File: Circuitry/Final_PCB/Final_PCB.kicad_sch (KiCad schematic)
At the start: 110 parts, among them Q1 Q_Dual_NMOS_S1G1D2S2G2D1, Q2 Q_Dual_NMOS_S1G1D2S2G2D1, Q3 Q_Dual_NMOS_S1G1D2S2G2D1, Q4 Q_Dual_NMOS_S1G1D2S2G2D1, Q5 Q_Dual_NMOS_S1G1D2S2G2D1, Q6 Q_Dual_NMOS_S1G1D2S2G2D1, Q7 Q_Dual_NMOS_S1G1D2S2G2D1, Q8 Q_Dual_NMOS_S1G1D2S2G2D1, SW1 SW_SPST, SW2 SW_SPST

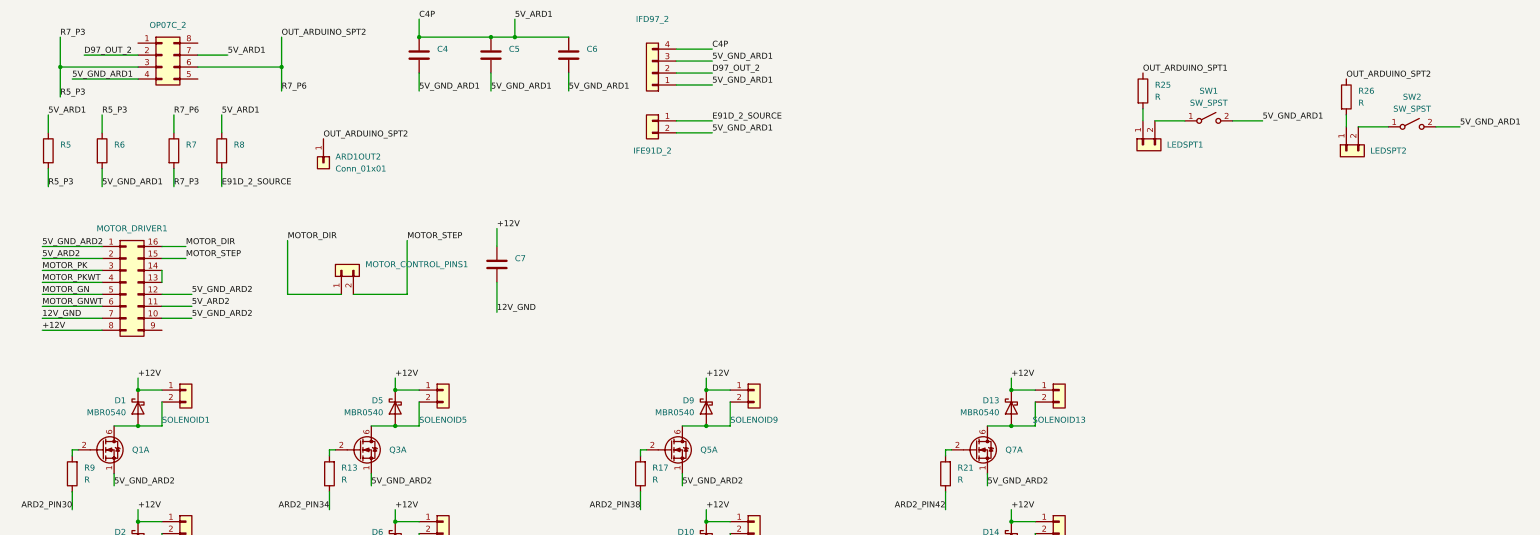
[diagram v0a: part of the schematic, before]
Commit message: final pcb and code updates
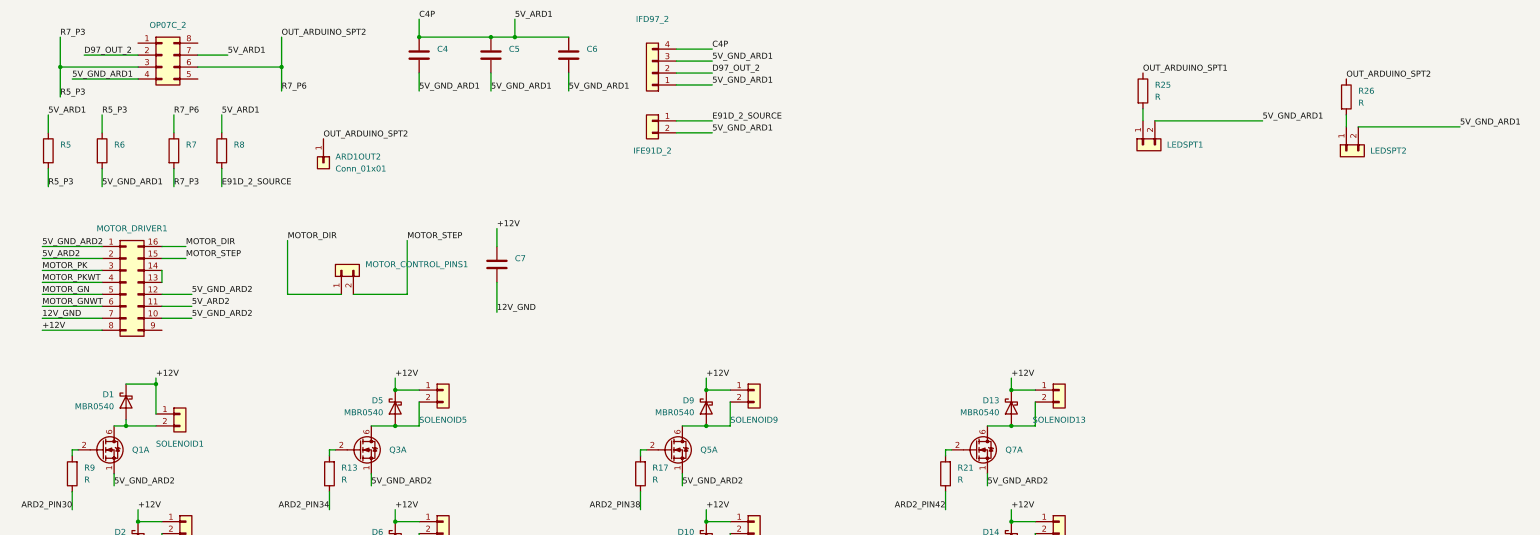
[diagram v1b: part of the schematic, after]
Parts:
- removed SW1, SW2: SW_SPST, Resistor_THT:R_Axial_DIN0207_L6.3mm_D2.5mm_P5.08mm_Vertical, symbol Switch:SW_SPST
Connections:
- net 12V_GND: now also LEDSPT1.2 (Pin_2), LEDSPT2.2 (Pin_2)
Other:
- moved on the sheet: SOLENOID1
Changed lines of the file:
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@@
   (junction (at 372.11 332.74) (diameter 0) (color 0 0 0 0)
   )
+  (junction (at 313.69 247.65) (diameter 0) (color 0 0 0 0)
+  )
   (junction (at 372.11 304.8) (diameter 0) (color 0 0 0 0)
   )
@@
   (junction (at 370.84 247.65) (diameter 0) (color 0 0 0 0)
   )
-  (junction (at 316.23 247.65) (diameter 0) (color 0 0 0 0)
-  )
-  (junction (at 316.23 240.03) (diameter 0) (color 0 0 0 0)
-  )
   (junction (at 502.92 304.8) (diameter 0) (color 0 0 0 0)
   )
@@
   (junction (at 436.88 247.65) (diameter 0) (color 0 0 0 0)
   )
+  (junction (at 320.04 238.76) (diameter 0) (color 0 0 0 0)
+  )
   (junction (at 519.43 143.51) (diameter 0) (color 0 0 0 0)
   )
@@
     (stroke (width 0) (type default))
   )
+  (wire (pts (xy 313.69 238.76) (xy 320.04 238.76))
+    (stroke (width 0) (type default))
+  )
   (wire (pts (xy 295.91 222.25) (xy 308.61 222.25))
     (stroke (width 0) (type default))
@@
     (stroke (width 0) (type default))
   )
-  (wire (pts (xy 316.23 240.03) (xy 321.31 240.03))
+  (wire (pts (xy 320.04 238.76) (xy 320.04 245.11))
     (stroke (width 0) (type default))
   )
@@
     (stroke (width 0) (type default))
   )
-  (wire (pts (xy 548.64 182.88) (xy 554.99 182.88))
-    (stroke (width 0) (type default))
-  )
   (wire (pts (xy 317.5 304.8) (xy 322.58 304.8))
     (stroke (width 0) (type default))
@@
     (stroke (width 0) (type default))
   )
-  (wire (pts (xy 581.66 184.15) (xy 575.31 184.15))
-    (stroke (width 0) (type default))
-  )
   (wire (pts (xy 347.98 123.19) (xy 347.98 129.54))
     (stroke (width 0) (type default))
@@
     (stroke (width 0) (type default))
   )
-  (wire (pts (xy 316.23 247.65) (xy 321.31 247.65))
-    (stroke (width 0) (type default))
-  )
   (wire (pts (xy 488.95 311.15) (xy 488.95 309.88))
     (stroke (width 0) (type default))
@@
     (stroke (width 0) (type default))
   )
+  (wire (pts (xy 313.69 247.65) (xy 320.04 247.65))
+    (stroke (width 0) (type default))
+  )
   (wire (pts (xy 496.57 275.59) (xy 501.65 275.59))
     (stroke (width 0) (type default))
@@
     (stroke (width 0) (type default))
   )
-  (wire (pts (xy 311.15 247.65) (xy 316.23 247.65))
+  (wire (pts (xy 311.15 247.65) (xy 313.69 247.65))
     (stroke (width 0) (type default))
   )
@@
     (stroke (width 0) (type default))
   )
-  (wire (pts (xy 591.82 184.15) (xy 596.9 184.15))
+  (wire (pts (xy 575.31 184.15) (xy 596.9 184.15))
     (stroke (width 0) (type default))
   )
@@
     (stroke (width 0) (type default))
   )
-  (wire (pts (xy 538.48 182.88) (xy 532.13 182.88))
+  (wire (pts (xy 532.13 182.88) (xy 554.99 182.88))
     (stroke (width 0) (type default))
   )
@@
     (stroke (width 0) (type default))
   )
-  (wire (pts (xy 316.23 237.49) (xy 316.23 240.03))
+  (wire (pts (xy 320.04 237.49) (xy 320.04 238.76))
     (stroke (width 0) (type default))
   )
@@
     (stroke (width 0) (type default))
   )
-  (wire (pts (xy 321.31 247.65) (xy 321.31 242.57))
-    (stroke (width 0) (type default))
-  )
   (wire (pts (xy 334.01 193.04) (xy 334.01 196.85))
     (stroke (width 0) (type default))
@@
     (stroke (width 0) (type default))
   )
+  (wire (pts (xy 313.69 246.38) (xy 313.69 247.65))
+    (stroke (width 0) (type default))
+  )
   (wire (pts (xy 424.18 281.94) (xy 424.18 280.67))
     (stroke (width 0) (type default))
@@
     (effects (font (size 1.27 1.27)) (justify left bottom))
   )
-  (label "+12V" (at 316.23 237.49 0) (fields_autoplaced)
+  (label "+12V" (at 320.04 237.49 0) (fields_autoplaced)
     (effects (font (size 1.27 1.27)) (justify left bottom))
   )
@@
     )
   )
-  (symbol (lib_id "Diode:MBR0540") (at 316.23 243.84 90) (mirror x) (unit 1)
-    (in_bom yes) (on_board yes) (dnp no)
-    (property "Reference" "D1" (at 313.69 242.2525 90)
-      (effects (font (size 1.27 1.27)) (justify left))
-    )
-    (property "Value" "MBR0540" (at 313.69 244.7925 90)
-      (effects (font (size 1.27 1.27)) (justify left))
-    )
-    (property "Footprint" "Diode_SMD:D_SOD-123" (at 320.675 243.84 0)
-      (effects (font (size 1.27 1.27)) hide)
-    )
-    (property "Datasheet" "http://www.mccsemi.com/up_pdf/MBR0520~MBR0580(SOD123).pdf" (at 316.23 243.84 0)
-      (effects (font (size 1.27 1.27)) hide)
-    )
-    (pin "1")
-    (pin "2")
-    (instances
-      (project "Final_PCB"
-        (path "/3aa8d99f-bc88-4d2c-936c-bff7aa7008c1"
-          (reference "D1") (unit 1)
-        )
-      )
-    )
-  )
   (symbol (lib_id "Connector_Generic:Conn_02x08_Counter_Clockwise") (at 313.69 217.17 0) (unit 1)
     (in_bom yes) (on_board yes) (dnp no) (fields_autoplaced)
@@
     )
   )
-  (symbol (lib_id "Connector_Generic:Conn_01x02") (at 326.39 240.03 0) (unit 1)
+  (symbol (lib_id "Connector_Generic:Conn_01x02") (at 325.12 245.11 0) (unit 1)
     (in_bom yes) (on_board yes) (dnp no)
-    (property "Reference" "SOLENOID1" (at 326.39 246.38 0)
+    (property "Reference" "SOLENOID1" (at 325.12 251.46 0)
       (effects (font (size 1.27 1.27)))
     )
-    (property "Value" "Conn_01x02" (at 325.12 245.11 90)
+    (property "Value" "Conn_01x02" (at 323.85 250.19 90)
       (effects (font (size 1.27 1.27)) (justify right) hide)
     )
-    (property "Footprint" "Resistor_THT:R_Axial_DIN0207_L6.3mm_D2.5mm_P5.08mm_Vertical" (at 326.39 240.03 0)
+    (property "Footprint" "Resistor_THT:R_Axial_DIN0207_L6.3mm_D2.5mm_P5.08mm_Vertical" (at 325.12 245.11 0)
       (effects (font (size 1.27 1.27)) hide)
     )
-    (property "Datasheet" "~" (at 326.39 240.03 0)
+    (property "Datasheet" "~" (at 325.12 245.11 0)
       (effects (font (size 1.27 1.27)) hide)
     )
@@
     )
   )
-  (symbol (lib_id "Switch:SW_SPST") (at 586.74 184.15 0) (unit 1)
-    (in_bom yes) (on_board yes) (dnp no)
-    (property "Reference" "SW2" (at 586.74 177.8 0)
-      (effects (font (size 1.27 1.27)))
-    )
-    (property "Value" "SW_SPST" (at 586.74 180.34 0)
-      (effects (font (size 1.27 1.27)))
-    )
-    (property "Footprint" "Resistor_THT:R_Axial_DIN0207_L6.3mm_D2.5mm_P5.08mm_Vertical" (at 586.74 184.15 0)
-      (effects (font (size 1.27 1.27)) hide)
-    )
-    (property "Datasheet" "~" (at 586.74 184.15 0)
-      (effects (font (size 1.27 1.27)) hide)
-    )
-    (pin "1")
-    (pin "2")
-    (instances
-      (project "Final_PCB"
-        (path "/3aa8d99f-bc88-4d2c-936c-bff7aa7008c1"
-          (reference "SW2") (unit 1)
-        )
-      )
-    )
-  )
   (symbol (lib_id "Connector_Generic:Conn_01x01") (at 330.2 365.76 270) (unit 1)
     (in_bom yes) (on_board yes) (dnp no) (fields_autoplaced)
@@
     )
   )
-  (symbol (lib_id "Switch:SW_SPST") (at 543.56 182.88 0) (unit 1)
-    (in_bom yes) (on_board yes) (dnp no) (fields_autoplaced)
-    (property "Reference" "SW1" (at 543.56 176.53 0)
-      (effects (font (size 1.27 1.27)))
-    )
-    (property "Value" "SW_SPST" (at 543.56 179.07 0)
-      (effects (font (size 1.27 1.27)))
-    )
-    (property "Footprint" "Resistor_THT:R_Axial_DIN0207_L6.3mm_D2.5mm_P5.08mm_Vertical" (at 543.56 182.88 0)
-      (effects (font (size 1.27 1.27)) hide)
-    )
-    (property "Datasheet" "~" (at 543.56 182.88 0)
-      (effects (font (size 1.27 1.27)) hide)
-    )
-    (pin "1")
-    (pin "2")
-    (instances
-      (project "Final_PCB"
-        (path "/3aa8d99f-bc88-4d2c-936c-bff7aa7008c1"
-          (reference "SW1") (unit 1)
-        )
-      )
-    )
-  )
   (symbol (lib_id "Diode:MBR0540") (at 372.11 328.93 90) (mirror x) (unit 1)
     (in_bom yes) (on_board yes) (dnp no)
@@
         )
       )
+    )
+  )
+  (symbol (lib_id "Diode:MBR0540") (at 313.69 242.57 90) (mirror x) (unit 1)
+    (in_bom yes) (on_board yes) (dnp no)
+    (property "Reference" "D1" (at 311.15 240.9825 90)
+      (effects (font (size 1.27 1.27)) (justify left))
+    )
+    (property "Value" "MBR0540" (at 311.15 243.5225 90)
+      (effects (font (size 1.27 1.27)) (justify left))
+    )
+    (property "Footprint" "Diode_SMD:D_SOD-123" (at 318.135 242.57 0)
+      (effects (font (size 1.27 1.27)) hide)
+    )
+    (property "Datasheet" "http://www.mccsemi.com/up_pdf/MBR0520~MBR0580(SOD123).pdf" (at 313.69 242.57 0)
+      (effects (font (size 1.27 1.27)) hide)
+    )
+    (pin "1")
+    (pin "2")
+    (instances
+      (project "Final_PCB"
+        (path "/3aa8d99f-bc88-4d2c-936c-bff7aa7008c1"
+          (reference "D1") (unit 1)
+        )
+      )
